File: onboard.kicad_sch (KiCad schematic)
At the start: 13 parts, among them Q2 2N7002K, Q3 2N7002K, SW3 SW_DIP_x08, SW4 User, U6 HDSM-293L

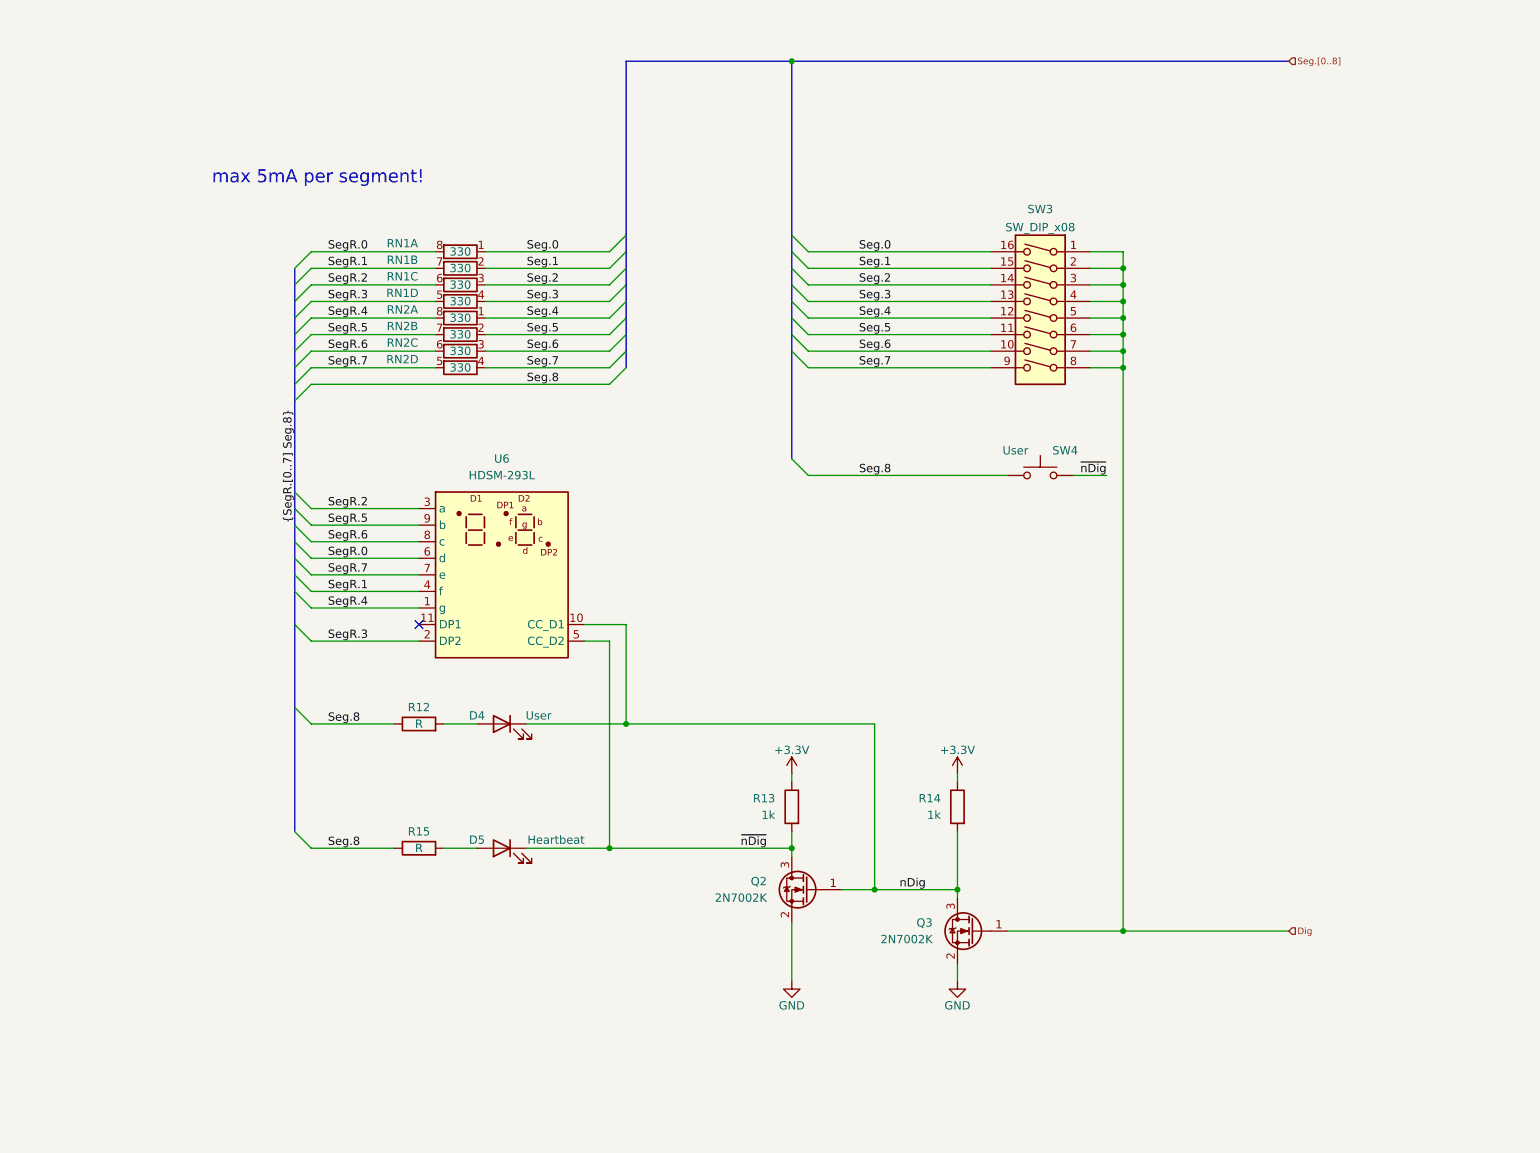
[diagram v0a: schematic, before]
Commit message: things changed
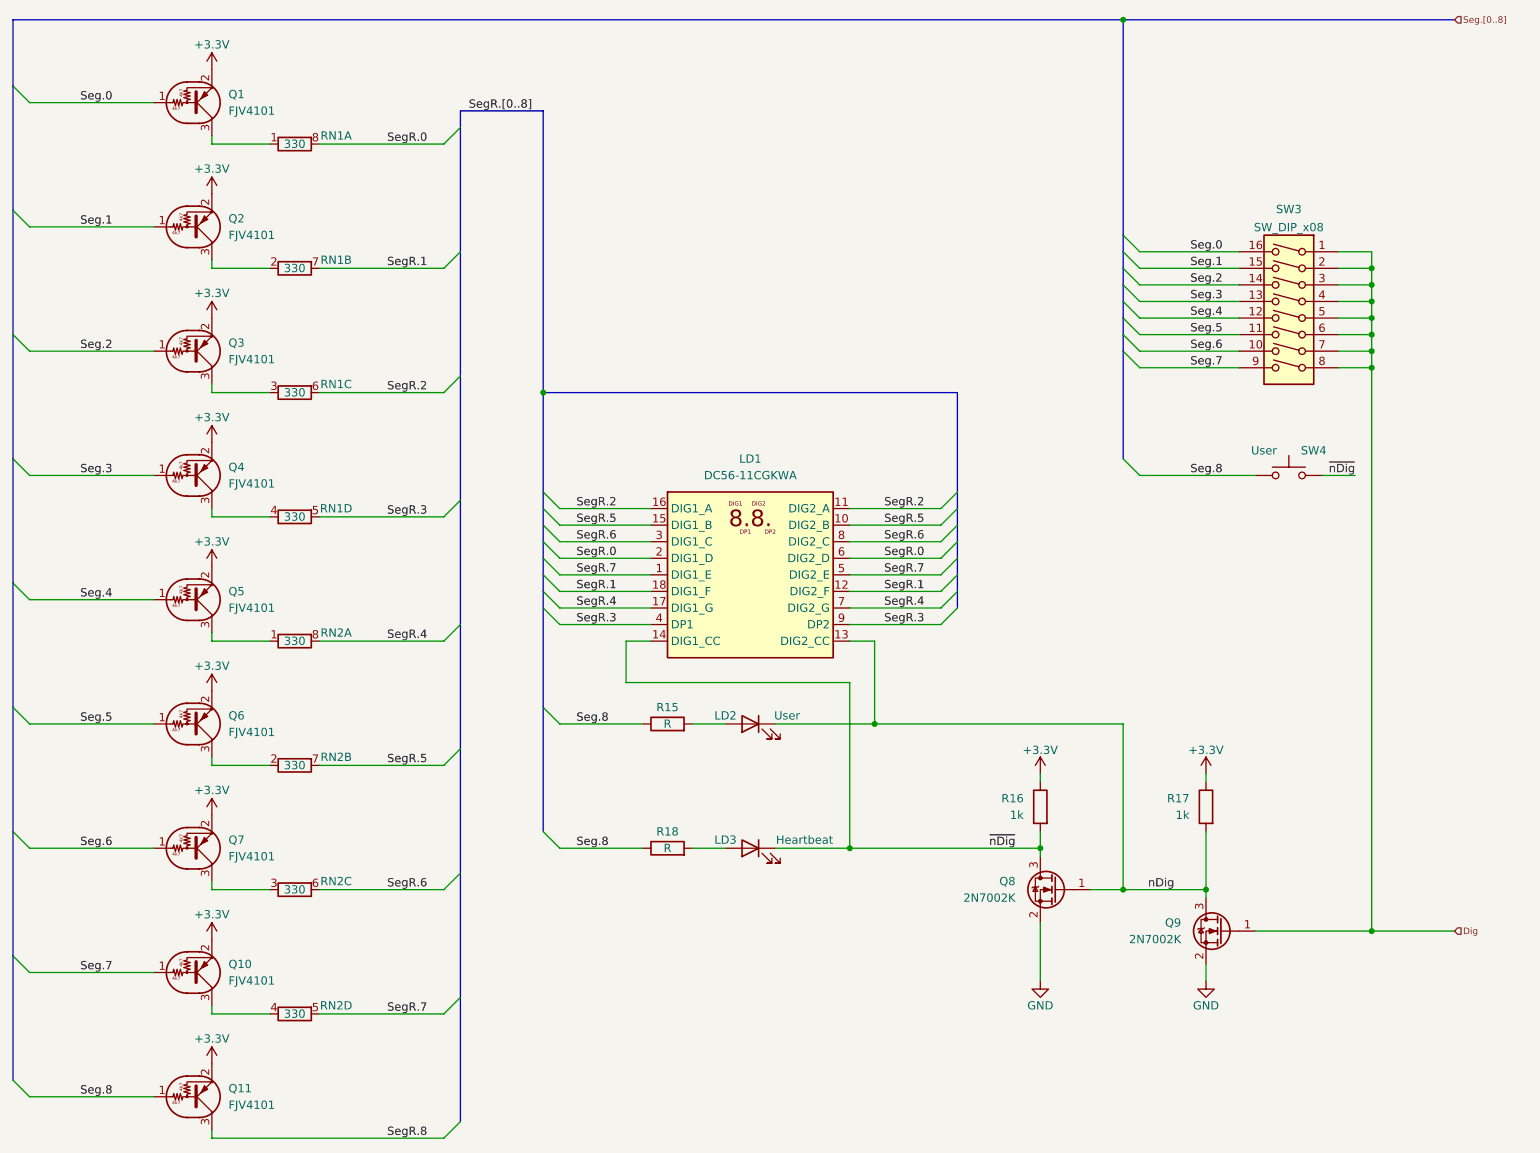
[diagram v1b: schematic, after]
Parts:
- removed U6: HDSM-293L, HDSM-293L:HDSM-293L, symbol HDSM-293L:HDSM-293L
- added LD1: DC56-11CGKWA, LB-402:LB-402, symbol Display_Character:DC56-11CGKWA
- added Q1, Q10, Q11, Q2, Q3, Q4, Q5, Q6, Q7: FJV4101, Package_TO_SOT_SMD:SOT-23, symbol Transistor_BJT:DTA143E
- renumbered D4 to LD2, D5 to LD3, Q2 to Q8, Q3 to Q9, R12 to R15, R13 to R16, R14 to R17, R15 to R18
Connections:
- net +3V3: now also Q1.2 (E), Q10.2 (E), Q11.2 (E), Q2.2 (E), Q3.2 (E), Q4.2 (E), Q5.2 (E), Q6.2 (E), Q7.2 (E)
- net Seg.0: now also Q1.1 (B); no longer RN1.1 (R1.1)
- net Seg.1: now also Q2.1 (B); no longer RN1.2 (R2.1)
- net Seg.2: now also Q3.1 (B); no longer RN1.3 (R3.1)
- net Seg.3: now also Q4.1 (B); no longer RN1.4 (R4.1)
- net Seg.4: now also Q5.1 (B); no longer RN2.1 (R1.1)
- net Seg.5: now also Q6.1 (B); no longer RN2.2 (R2.1)
- net Seg.6: now also Q7.1 (B); no longer RN2.3 (R3.1)
- net Seg.7: now also Q10.1 (B); no longer RN2.4 (R4.1)
- net Seg.8: now also Q11.1 (B)
- net SegR.0: now also LD1.2 (DIG1_D), LD1.6 (DIG2_D)
- net SegR.1: now also LD1.12 (DIG2_F), LD1.18 (DIG1_F)
- net SegR.2: now also LD1.11 (DIG2_A), LD1.16 (DIG1_A)
- net SegR.3: now also LD1.4 (DP1), LD1.9 (DP2)
- net SegR.4: now also LD1.17 (DIG1_G), LD1.7 (DIG2_G)
- net SegR.5: now also LD1.10 (DIG2_B), LD1.15 (DIG1_B)
- net SegR.6: now also LD1.3 (DIG1_C), LD1.8 (DIG2_C)
- net SegR.7: now also LD1.1 (DIG1_E), LD1.5 (DIG2_E)
- net nDig: now also LD1.13 (DIG2_CC)
- net ~{nDig}: now also LD1.14 (DIG1_CC)
- new net: Q4.3 (C), RN1.4 (R4.1)
- new net: Q5.3 (C), RN2.1 (R1.1)
- new net: Q6.3 (C), RN2.2 (R2.1)
- new net: Q2.3 (C), RN1.2 (R2.1)
- new net: Q1.3 (C), RN1.1 (R1.1)
- new net: Q7.3 (C), RN2.3 (R3.1)
- new net: Q3.3 (C), RN1.3 (R3.1)
- new net: Q10.3 (C), RN2.4 (R4.1)
- new net SegR.8: Q11.3 (C)
- no-connect marks 1 -> 0
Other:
- note removed: "max 5mA per segment!"
- moved on the sheet: LD2, LD3, Q8, Q9, R15, R16, R17, R18, RN1A, RN1B, RN1C, RN1D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
